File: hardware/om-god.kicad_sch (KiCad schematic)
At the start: 0 parts

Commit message: fd
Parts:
- added C1: 100nF, Capacitor_SMD:C_0402_1005Metric, symbol Device:C
- added C44, C55, C59, C60, C61, C62, C70, C71: 10uF, Capacitor_SMD:C_0402_1005Metric, symbol Device:C
- added C45: 22uF, Capacitor_SMD:C_0402_1005Metric, symbol Device:C
- added C56, C65, C66: 1uF, Capacitor_SMD:C_0402_1005Metric, symbol Device:C
- added C57, C69: 4.7uF, Capacitor_SMD:C_0402_1005Metric, symbol Device:C
- added C58: 47nF, Capacitor_SMD:C_0402_1005Metric, symbol Device:C
- added C63, C67, C68: 2.2uF, Capacitor_SMD:C_0402_1005Metric, symbol Device:C
- added C64: 470nF, Capacitor_SMD:C_0402_1005Metric, symbol Device:C
- added CN1: USB-B-Female-90, lcsc:USB-B_TH_USB-B-FEMALE-90, symbol lcsc:USB-B-Female-90
- added CN2, CN3: DIN-504B-M10, lcsc:CONN-TH_DIN-504B-M10, symbol lcsc:DIN-504B-M10
- added CN4: PJ-320D, lcsc:AUDIO-SMD_PJ-320D, symbol lcsc:PJ-320D
- added Card1: TF PUSH, lcsc:TF-SMD_TF-PUSH, symbol lcsc:TFPUSH
- added D1, D10, D11, D12, D13, D14, D15, D16, D17, D18, D19, D2, D20, D21, D22, D23, D24, D25, D3, D4, D5, D50, D51, D52, D53, D54, D55, D56, D57, D58, D59, D6, D60, D61, D62, D63, D64, D65, D66, D67, D68, D69, D7, D70, D71, D72, D8, D9: 1N4148WS_C917117, lcsc:SOD-323_L1.8-W1.3-LS2.5-RD, symbol lcsc:1N4148WS_C917117
- added D26: 1N4148WT, Diode_SMD:D_SOD-523, symbol Diode:1N4148WT
- added D27: PESD15VL1BA, PCM_Diode_SMD_AKL:D_SOD-323_TVS, symbol PCM_Diode_TVS_AKL:PESD15VL1BA
- added FPC1: 5034801200, lcsc:FPC-SMD_5034801200, symbol lcsc:5034801200
- added J1, J2: Conn_01x13_Pin, symbol Connector:Conn_01x13_Pin
- added J3, J4, J5: PJ-625G, lcsc:AUDIO-TH_PJ-625G, symbol lcsc:PJ-625G
- added J6, J7: Conn_01x01_Pin, symbol Connector:Conn_01x01_Pin
- added J8: Conn_01x03, Connector_JST:JST_EH_S3B-EH_1x03_P2.50mm_Horizontal, symbol Connector_Generic:Conn_01x03
- added L4: 1uH, Inductor_SMD:L_0603_1608Metric, symbol Device:L
- added L5, L6: 470nH, Inductor_SMD:L_0603_1608Metric, symbol Device:L
- added L8: EXC14CE900U, linea:FILTER-SMD_4P-L0.9-W0.7-P0.50-BL, symbol linea:EXC14CE900U
- added L9: 470nH, Inductor_SMD:L_Murata_DFE201610P, symbol Device:L
- added Q4: ~, linea:SOT-523-3_L1.6-W0.8-P1.00-LS1.6-BR, symbol DMN313DLT-7:DMN313DLT-7
- added Q5: ~, linea:SOT-363_L2.0-W1.3-P0.65-LS2.1-BL, symbol MMDT2907A-7-F:MMDT2907A-7-F
- added Q6: ~, linea:SOT-23-3_L2.9-W1.3-P1.90-LS2.4-BR, symbol DMP1045U-7:DMP1045U-7
- added R1, R2: 5.1K, Resistor_SMD:R_0402_1005Metric, symbol Device:R
- added R31, R32: 1.5K, Resistor_SMD:R_0402_1005Metric, symbol Device:R
- added R33: 4.7K, Resistor_SMD:R_0402_1005Metric, symbol Device:R
- added R34, R36, R40, R41: 10K, Resistor_SMD:R_0402_1005Metric, symbol Device:R
- added R35: 100, Resistor_SMD:R_0402_1005Metric, symbol Device:R
- added R37: 470, Resistor_SMD:R_0402_1005Metric, symbol Device:R
- added R38: 30.1K, Resistor_SMD:R_0402_1005Metric, symbol Device:R
- added R39: 5.23K, Resistor_SMD:R_0402_1005Metric, symbol Device:R
- added R42: 10m, Resistor_SMD:R_0402_1005Metric, symbol Device:R
- added R43: DNP, Resistor_SMD:R_0402_1005Metric, symbol Device:R
- added R44, R45: 1.5, Resistor_SMD:R_0402_1005Metric, symbol Device:R
- added R46, R47: 3.3, Resistor_SMD:R_0402_1005Metric, symbol Device:R
- added R48, R49: 100K, Resistor_SMD:R_0402_1005Metric, symbol Device:R
- added SW1, SW10, SW11, SW12, SW13, SW14, SW15, SW16, SW17, SW18, SW19, SW2, SW20, SW21, SW22, SW23, SW24, SW25, SW26, SW27, SW28, SW29, SW3, SW30, SW31, SW32, SW33, SW34, SW35, SW36, SW37, SW38, SW39, SW4, SW40, SW41, SW42, SW43, SW44, SW45, SW46, SW47, SW48, SW5, SW56, SW57, SW58, SW6, SW7, SW8, SW9: TS-1003ST-26, lcsc:SW-SMD_4P-L12.0-W12.0-P5.00-LS15.4, symbol lcsc:TS-1003ST-26
- added SW49: RotaryEncoder_Switch, symbol Device:RotaryEncoder_Switch
- added SW50, SW51, SW52, SW53, SW54, SW55: RotaryEncoder, symbol Device:RotaryEncoder
- added TP1, TP2, TP3: TestPoint, TestPoint:TestPoint_Pad_1.5x1.5mm, symbol Connector:TestPoint
- added U1: TDA7297, Package_TO_SOT_THT:TO-220-15_P2.54x2.54mm_StaggerOdd_Lead4.58mm_Vertical, symbol Amplifier_Audio:TDA7297
- added U10, U11, U7, U8, U9: ~, lcsc:SW-TH_6P-L8.0-W8.0-P2.50, symbol lcsc:XKB8080-Z
- added U12: ~, linea:DSBGA-6_L1.4-W1.1-R3-C2-P0.40-BL, symbol LM3281YFQR:LM3281YFQR
- added U13: ~, linea:QFN-24_L4.0-W4.0-P0.50-TL-EP2.7, symbol BQ25896RTWR:BQ25896RTWR
- added U14: ~, linea:DSBGA-9_L1.7-W1.6-R3-C3-P0.50-BL, symbol BQ27220YZFR:BQ27220YZFR
- added U15: FAN48610BUC50X, linea:WLCSP-9_L1.2-W1.2-R3-C3-P0.40-BL, symbol linea:FAN48610BUC50X
- added U16: RS3221-3.3YUTDN4, linea:UTDFN-4_L1.0-W1.0-P0.63-BL-EP-1, symbol linea:RS3221-3.3YUTDN4
- added U17: USBLC6-2P6, Package_TO_SOT_SMD:SOT-666, symbol Power_Protection:USBLC6-2P6
- added U2: TPA3116D2DAD_C2865736, lcsc:HTSSOP-32_L11.0-W6.1-P0.65-LS8.1-BL, symbol lcsc:TPA3116D2DAD_C2865736
- added U3: CY8CMBR3116-LQXIT, lcsc:QFN-24_L4.0-W4.0-P0.50-BL-EP2.6, symbol lcsc:CY8CMBR3116-LQXIT
- added U4: PCM5102APWR, lcsc:TSSOP-20_L6.5-W4.4-P0.65-LS6.4-BL, symbol lcsc:PCM5102APWR
- added U5: HS20HS072RX, lcsc:OLED-SMD_HS20HS072RX, symbol lcsc:HS20HS072RX
- added U6: MKDV4GCL-ABB, lcsc:LGA-8_L6.0-W8.0-P1.27-TL, symbol lcsc:MKDV4GCL-ABB
- added USB2: TYPE-C 16PIN 2MD(073), linea:USB-C-SMD_TYPE-C-6PIN-2MD-073, symbol linea:TYPE-C16PIN2MD(073)
- added VQ: STM32H723ZGT6, lcsc:LQFP-144_L20.0-W20.0-P0.50-LS22.0-BL, symbol lcsc:STM32H723ZGT6
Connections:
- new net: D72.2 (A), SW23.1, SW23.2
- new net: D52.2 (A), SW2.1, SW2.2
- new net: D70.2 (A), SW21.1, SW21.2
- new net: D21.2 (A), SW44.1, SW44.2
- new net: D3.2 (A), SW26.1, SW26.2
- new net: D60.2 (A), SW10.1, SW10.2
- new net: D65.2 (A), SW16.1, SW16.2
- new net: D2.2 (A), SW24.1, SW24.2
- new net: D19.2 (A), SW42.1, SW42.2
- new net: L8.3, U17.6 (I/O1)
- new net: L8.4, U17.4 (I/O2)
- new net: D57.2 (A), SW7.1, SW7.2
- new net: Q5.3 (C2), R48.1
- new net: D24.2 (A), SW47.1, SW47.2
- new net: D63.2 (A), SW14.1, SW14.2
- new net: C68.1, C69.1, C70.1, L6.1, R44.1, R45.1, U12.A1 (FB)
- new net: L5.1, U12.B2 (SW)
- new net: L6.2, R46.2, R47.2
- new net: L5.2, R44.2, R45.2
- new net: D5.2 (A), SW28.1, SW28.2
- new net: D61.2 (A), SW11.1, SW11.2
- new net: D9.2 (A), SW32.1, SW32.2
- new net: D56.2 (A), SW6.1, SW6.2
- new net: D64.2 (A), SW15.1, SW15.2
- new net: D12.2 (A), SW35.1, SW35.2
- new net: L9.2, U15.B1 (SW), U15.B2 (SW)
- new net: D20.2 (A), SW43.1, SW43.2
- new net: D17.2 (A), SW40.1, SW40.2
- new net: R37.2, U13.10 (LIIM)
- new net: J8.2 (Pin_2), R38.2, R39.2, R43.1, TP2.1, U13.11 (TS)
- new net: C61.1, C62.1, C66.1, R42.2, U13.13 (BAT), U13.14 (BAT), U14.C2 (SRN), U16.3 (EN), U16.4 (IN)
- new net: C58.1, L4.1, U13.19 (SW), U13.20 (SW)
- new net: C58.2, U13.21 (BTST)
- new net: C57.1, R39.1, U13.22 (REGN)
- new net: C55.1, U13.23 (PMID)
- new net: R33.1, U13.7 (INT)
- new net: Q4.3 (D), R34.1, U13.8 (OTG)
- new net: D13.2 (A), SW36.1, SW36.2
- new net: Q4.1 (G), R35.1, R36.2
- new net: D62.2 (A), SW12.1, SW12.2
- new net: D55.2 (A), SW5.1, SW5.2
- new net: D51.2 (A), SW25.1, SW25.2
- new net: D16.2 (A), SW39.1, SW39.2
- new net: D23.2 (A), SW46.1, SW46.2
- new net: D7.2 (A), SW30.1, SW30.2
- new net: R2.1, USB2.10 (CC2)
- new net: D11.2 (A), SW34.1, SW34.2
- new net: D68.2 (A), SW19.1, SW19.2
- new net: D14.2 (A), SW37.1, SW37.2
- new net: D15.2 (A), SW38.1, SW38.2
- new net: D8.2 (A), SW31.1, SW31.2
- new net: D54.2 (A), SW4.1, SW4.2
- new net: D53.2 (A), SW3.1, SW3.2
- new net: R40.1, U14.A1 (GPOUT)
- new net: R41.2, U14.B1 (BIN)
- new net: C63.1, C64.1, U14.B3 (VDD)
- new net: D66.2 (A), SW17.1, SW17.2
- new net: D18.2 (A), SW41.1, SW41.2
- new net: D22.2 (A), SW45.1, SW45.2
- new net: D50.2 (A), SW13.1, SW13.2
- new net: D26.2 (A), Q5.2 (B1), Q5.5 (B2)
- new net: Q5.6 (C1), Q6.1 (G), R49.1
- new net: D67.2 (A), SW18.1, SW18.2
- new net: D25.2 (A), SW48.1, SW48.2
- new net: D59.2 (A), SW9.1, SW9.2
- new net: U17.1 (I/O1), USB2.6 (DP1), USB2.8 (DP2)
- new net: U17.3 (I/O2), USB2.5 (DN2), USB2.7 (DN1)
- new net: D1.2 (A), SW1.1, SW1.2
- new net: D10.2 (A), SW33.1, SW33.2
- new net: D58.2 (A), SW8.1, SW8.2
- new net: R1.1, USB2.4 (CC1)
- new net: D6.2 (A), SW29.1, SW29.2
- new net: D71.2 (A), SW22.1, SW22.2
- new net: D69.2 (A), SW20.1, SW20.2
- new net: D4.2 (A), SW27.1, SW27.2
- new net +3.3V: C71.1, R31.2, R32.2, R33.2, R40.2, R46.1, R47.1
- new net +5V: C45.1, U15.A1 (VOUT), U15.A2 (VOUT)
- new net +BATT: C65.1, J8.1 (Pin_1), R42.1, TP1.1, U14.C1 (SRP), U14.C3 (BAT)
- new net 7th: D10.1 (C), D12.1 (C), D14.1 (C), D16.1 (C), D18.1 (C), D2.1 (C), D20.1 (C), D22.1 (C), D24.1 (C), D4.1 (C), D6.1 (C), D8.1 (C)
- new net Chord A: SW1.3, SW1.4, SW11.3, SW11.4, SW24.3, SW24.4, SW26.3, SW26.4
- new net Chord Ab: SW10.3, SW10.4, SW23.3, SW23.4, SW47.3, SW47.4, SW48.3, SW48.4
- new net Chord B: SW14.3, SW14.4, SW25.3, SW25.4, SW29.3, SW29.4, SW30.3, SW30.4
- new net Chord Bb: SW12.3, SW12.4, SW13.3, SW13.4, SW27.3, SW27.4, SW28.3, SW28.4
- new net Chord C: SW15.3, SW15.4, SW2.3, SW2.4, SW31.3, SW31.4, SW32.3, SW32.4
- new net Chord D: SW17.3, SW17.4, SW35.3, SW35.4, SW36.3, SW36.4, SW4.3, SW4.4
- new net Chord Db: SW16.3, SW16.4, SW3.3, SW3.4, SW33.3, SW33.4, SW34.3, SW34.4
- new net Chord E: SW19.3, SW19.4, SW39.3, SW39.4, SW40.3, SW40.4, SW6.3, SW6.4
- new net Chord Eb: SW18.3, SW18.4, SW37.3, SW37.4, SW38.3, SW38.4, SW5.3, SW5.4
- new net Chord F: SW20.3, SW20.4, SW41.3, SW41.4, SW42.3, SW42.4, SW7.3, SW7.4
- new net Chord G: SW22.3, SW22.4, SW45.3, SW45.4, SW46.3, SW46.4, SW9.3, SW9.4
- new net Chord Gb: SW21.3, SW21.4, SW43.3, SW43.4, SW44.3, SW44.4, SW8.3, SW8.4
- new net Extention: D11.1 (C), D13.1 (C), D15.1 (C), D17.1 (C), D19.1 (C), D21.1 (C), D23.1 (C), D25.1 (C), D3.1 (C), D5.1 (C), D7.1 (C), D9.1 (C)
- new net GND: C1.2, C44.2, C45.2, C55.2, C56.2, C57.2, C59.2, C60.2, C61.2, C62.2, C63.2, C64.2, C65.2, C66.2, C67.2, C68.2, C69.2, C70.2, C71.2, D27.1 (K), J8.3 (Pin_3), Q4.2 (S), R1.2, R2.2, R36.1, R37.1, R38.1, R41.1, R43.2, R48.2, R49.2, TP3.1, U12.C2 (GND), U13.17 (PGND), U13.18 (PGND), U13.2 (PSEL), U13.25 (EPAD), U13.9 (CE), U14.B2 (VSS), U15.C1 (PGND), U15.C2 (PGND), U15.C3 (AGND), U16.2 (GND), U16.5 (EP), U17.2 (GND), USB2.1 (GND), USB2.12 (GND), USB2.13 (SHELL), USB2.14 (SHELL)
- new net I2C_SCL: R31.1, U13.5 (SCL), U14.A3 (SCL)
- new net I2C_SDA: R32.1, U13.6 (SDA), U14.A2 (SDA)
- new net LDO_3.3V: U16.1 (OUT)
- new net Mayor: D1.1 (C), D50.1 (C), D51.1 (C), D52.1 (C), D53.1 (C), D54.1 (C), D55.1 (C), D56.1 (C), D57.1 (C), D58.1 (C), D59.1 (C), D60.1 (C)
- new net Minor: D61.1 (C), D62.1 (C), D63.1 (C), D64.1 (C), D65.1 (C), D66.1 (C), D67.1 (C), D68.1 (C), D69.1 (C), D70.1 (C), D71.1 (C), D72.1 (C)
- new net RESET: U13.12 (QON)
- new net SYS: C44.1, C59.1, C60.1, C67.1, L4.2, L9.1, R34.2, U12.A2 (VIN), U12.B1 (MODE), U12.C1 (EN), U13.15 (SYS), U13.16 (SYS), U15.A3 (VIN), U15.B3 (EN)
- new net USB_5V: C56.1, Q5.4 (E2), Q6.2 (S), U13.1 (VBUS)
- new net VBUS: C1.1, D26.1 (K), D27.2 (A), Q5.1 (E1), Q6.3 (D), R35.2, U17.5 (VBUS), USB2.11 (VBUS), USB2.2 (VBUS)
- no-connect marks 0 -> 3
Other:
- note added: "Advanced Funtionalities"
- note added: "Audio Amplifiers"
- note added: "Audio Out"
- note added: "Chord Matrix"
- note added: "Chords Volume"
- note added: "DAC"
- note added: "DIN-MIDI"
- note added: "External Micro SD Card"
- note added: "Function Knob"
- note added: "Headphones Out"
- note added: "I/O"
- note added: "If using thermistor, remove R43"
- note added: "Instant Off"
- note added: "Keyboard Volume"
- note added: "Main"
- note added: "Main Buttons"
- note added: "Main Knobs"
- note added: "Main Volume"
- note added: "Metronome"
- note added: "Midi"
- note added: "NAnd Flash"
- note added: "Next Chord"
- note added: "Octave Down"
- note added: "Octave Up"
- note added: "On/Off"
- note added: "Pedal"
- note added: "Power Managment"
- note added: "Recording"
- note added: "Recording Mode"
- note added: "Rythm"
- note added: "Rythm Volume"
- note added: "Sonic Strings"
- note added: "Stereo Out"
- note added: "Sustain Chord"
- note added: "Touch Pad"
- note added: "Touch Pad Volume"
- note added: "USB-MIDI"
- note added: "Usb Power outlet / Coding"
- note added: "VQ"
- note added: "Vibrato Knob"
- note added: "Volume"

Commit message: yes
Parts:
- removed CN4: PJ-320D, lcsc:AUDIO-SMD_PJ-320D, symbol lcsc:PJ-320D
- removed D26: 1N4148WT, Diode_SMD:D_SOD-523, symbol Diode:1N4148WT
- removed J2: Conn_01x13_Pin, symbol Connector:Conn_01x13_Pin
- removed J6, J7: Conn_01x01_Pin, symbol Connector:Conn_01x01_Pin
- removed J8: Conn_01x03, Connector_JST:JST_EH_S3B-EH_1x03_P2.50mm_Horizontal, symbol Connector_Generic:Conn_01x03
- removed L9: 470nH, Inductor_SMD:L_Murata_DFE201610P, symbol Device:L
- removed Q4: ~, linea:SOT-523-3_L1.6-W0.8-P1.00-LS1.6-BR, symbol DMN313DLT-7:DMN313DLT-7
- removed Q5: ~, linea:SOT-363_L2.0-W1.3-P0.65-LS2.1-BL, symbol MMDT2907A-7-F:MMDT2907A-7-F
- removed Q6: ~, linea:SOT-23-3_L2.9-W1.3-P1.90-LS2.4-BR, symbol DMP1045U-7:DMP1045U-7
- removed TP1, TP2, TP3: TestPoint, TestPoint:TestPoint_Pad_1.5x1.5mm, symbol Connector:TestPoint
- removed U1: TDA7297, Package_TO_SOT_THT:TO-220-15_P2.54x2.54mm_StaggerOdd_Lead4.58mm_Vertical, symbol Amplifier_Audio:TDA7297
- removed U12: ~, linea:DSBGA-6_L1.4-W1.1-R3-C2-P0.40-BL, symbol LM3281YFQR:LM3281YFQR
- removed U13: ~, linea:QFN-24_L4.0-W4.0-P0.50-TL-EP2.7, symbol BQ25896RTWR:BQ25896RTWR
- removed U14: ~, linea:DSBGA-9_L1.7-W1.6-R3-C3-P0.50-BL, symbol BQ27220YZFR:BQ27220YZFR
- removed U15: FAN48610BUC50X, linea:WLCSP-9_L1.2-W1.2-R3-C3-P0.40-BL, symbol linea:FAN48610BUC50X
- removed U16: RS3221-3.3YUTDN4, linea:UTDFN-4_L1.0-W1.0-P0.63-BL-EP-1, symbol linea:RS3221-3.3YUTDN4
- removed U4: PCM5102APWR, lcsc:TSSOP-20_L6.5-W4.4-P0.65-LS6.4-BL, symbol lcsc:PCM5102APWR
- added AUDIO1: PJ-393_C2837065, lcsc:AUDIO-SMD_PJ-393, symbol lcsc:PJ-393_C2837065
- added C10, C104, C12, C133, C134, C135, C136, C142, C143, C145, C146, C148, C155, C156, C157, C158, C167, C177, C179, C180, C181, C185, C186, C189, C19, C194, C20, C3, C4, C41, C42, C43, C46, C47, C48, C49, C5, C51, C52, C53, C54, C6, C7, C8, C82, C83, C84, C86, C9, C94, C96: 0.1uF, symbol Device:C
- added C105, C106, C107, C120, C121, C124, C127, C128, C166, C22, C23, C24, C32, C33, C34, C35, C50, C95: 1uF, symbol Device:C
- added C108, C109, C21, C25, C38: 1nF, symbol Device:C
- added C11, C18, C188, C191, C195, C196, C2, C80, C81, C85, C92, C93, C97: 2.2uF, symbol Device:C
- added C110, C111, C112, C113, C165, C28, C29, C30, C31: 220nF, symbol Device:C
- added C114, C115, C131, C26, C39: 100nF, symbol Device:C
- added C116, C117, C27, C40: 220uF, symbol Device:C_Polarized
- added C118, C119, C125, C126: 680nF, symbol Device:C
- added C122, C123, C129, C130, C132, C36, C37: 10nF, symbol Device:C
- added C13, C14, C147, C15, C150, C152, C153, C16, C17, C184, C187, C190, C192, C193, C87, C88, C89, C90, C91: 10uF, symbol Device:C_Polarized
- added C137, C138: 220pF, Capacitor_SMD:C_0402_1005Metric, symbol Device:C
- added C139: 0.1uF, Capacitor_SMD:C_0402_1005Metric, symbol Device:C
- added C140, C149, C151: 1uF, symbol Device:C_Polarized
- added C141: 0.056uF, symbol Device:C_Polarized
- added C144: 2.2uF, symbol Device:C_Polarized
- added C154: 22pF, symbol Device:C
- added C159, C168: 47pF, symbol Device:C
- added C160, C161, C162, C163, C169, C170, C171, C172, C173, C174, C182, C183: 22uF, symbol Device:C
- added C164, C175, C176, C178: 10uF, symbol Device:C
- added C72, C73, C75, C77: 82nF, PCM_Capacitor_THT_AKL:C_Rect_L4.0mm_W2.5mm_P2.50mm, symbol PCM_Capacitor_AKL:C_Rect_L4.0mm_W2.5mm_P2.50mm
- added C74, C76, C78, C79: 5.6nF, PCM_Capacitor_THT_AKL:C_Rect_L4.0mm_W2.5mm_P2.50mm, symbol PCM_Capacitor_AKL:C_Rect_L4.0mm_W2.5mm_P2.50mm
- added D28: BAT54, PCM_Package_TO_SOT_SMD_AKL:SOT-23, symbol PCM_Diode_Schottky_AKL:BAT54
- added D29, D30, D31: LED, symbol Device:LED
- added J2: Conn_01x03_Pin, symbol Connector:Conn_01x03_Pin
- added L1, L10, L11, L2, L3, L7: 10uH, symbol Device:L
- added L12: 6.8uH, Inductor_SMD:L_6.3x6.3_H3, symbol Device:L
- added L13: 6.8uH, symbol Device:L
- added L14: 15uH, symbol Device:L
- added Q1, Q2, Q3: Si7617DN, Package_SO:Vishay_PowerPAK_1212-8_Single, symbol Transistor_FET:Si7617DN
- added R10, R13, R17, R18, R26: 100k, symbol Device:R
- added R100, R101, R87, R99: 10K, Resistor_SMD:R_0402_1005Metric, symbol Device:R
- added R102, R66, R69, R74: 100K, Resistor_SMD:R_0402_1005Metric, symbol Device:R
- added R103: NTCG163JF103FT1S, lcsc:R0603, symbol lcsc:NTCG163JF103FT1S
- added R104: 9.31K, Resistor_SMD:R_0402_1005Metric, symbol Device:R
- added R105: 430K, Resistor_SMD:R_0402_1005Metric, symbol Device:R
- added R11, R16: 75k, symbol Device:R
- added R12, R9: 47k, symbol Device:R
- added R14, R15, R19, R20, R24, R25: 3.3, symbol Device:R
- added R21, R22, R27, R28, R29, R30, R50, R51, R52, R53, R7, R8, R82, R83, R84, R85: 10K, symbol Device:R
- added R23: 10k, symbol Device:R
- added R3, R4: 470K, symbol Device:R
- added R5, R59, R6, R60, R61, R62, R63, R64, R65, R67, R68, R70, R71, R72, R73, R75: 6K, symbol Device:R
- added R58: 200K, Resistor_SMD:R_0402_1005Metric, symbol Device:R
- added R76, R77, R78, R79, R80, R81, R89, R94: 1K, symbol Device:R
- added R86: 22.1K, Resistor_SMD:R_0402_1005Metric, symbol Device:R
- added R88: 32.4K, Resistor_SMD:R_0402_1005Metric, symbol Device:R
- added R90, R95, R98: 100K, symbol Device:R
- added R91: 10, symbol Device:R
- added R92: 2, symbol Device:R
- added R93, R96: 0.01, symbol Device:R
- added R97: 500K, symbol Device:R
- added U1, U18, U19, U20, U22, U24, U25, U28, U29: NE5532DR, lcsc:SOIC-8_L4.9-W3.9-P1.27-LS6.0-BL, symbol lcsc:NE5532DR
- added U12, U13, U14, U35: LMR33630ADDAR, lcsc:ESOP-8_L4.9-W3.9-P1.27-LS6.0-TL-EP, symbol lcsc:LMR33630ADDAR
- added U15: TPS54202DDC, Package_TO_SOT_SMD:SOT-23-6, symbol Regulator_Switching:TPS54202DDC
- added U16, U26, U4: PCM5122PW, Package_SO:TSSOP-28_4.4x9.7mm_P0.65mm, symbol Audio:PCM5122PW
- added U21: TPA6120A2DWP, lcsc:HSOP-20_L12.8-W7.5-P1.27-LS10.3-BL-EP3.3, symbol lcsc:TPA6120A2DWP
- added U23: TS5A23159RSER, lcsc:UQFN-10_L2.0-W1.5-P0.50-BL-EP, symbol lcsc:TS5A23159RSER
- added U30: TPA3116D2DAD_C2865736, lcsc:HTSSOP-32_L11.0-W6.1-P0.65-LS8.1-BL, symbol lcsc:TPA3116D2DAD_C2865736
- added U31: BQ24610, Package_DFN_QFN:VQFN-24-1EP_4x4mm_P0.5mm_EP2.45x2.45mm, symbol Battery_Management:BQ24610
- added U32: TUSB422IYFPR, lcsc:DSBGA-9_L1.4-W1.3-R3-C3-P0.40-BL, symbol lcsc:TUSB422IYFPR
- added U33, U34: SIS412DN-T1-GE3-ES, lcsc:PDFN-8_L3.1-W3.1-P0.65-LS3.4-BL, symbol lcsc:SIS412DN-T1-GE3-ES
- C44, C66: footprint Capacitor_SMD:C_0402_1005Metric -> (none)
- C45: value 22uF -> 220nF; footprint Capacitor_SMD:C_0402_1005Metric -> (none)
- C55: value 10uF -> 0.1uF; footprint Capacitor_SMD:C_0402_1005Metric -> (none)
- C56: value 1uF -> 47pF; footprint Capacitor_SMD:C_0402_1005Metric -> (none); now not fitted
- C57: value 4.7uF -> 22uF; footprint Capacitor_SMD:C_0402_1005Metric -> (none)
- C58: value 47nF -> 22uF; footprint Capacitor_SMD:C_0402_1005Metric -> (none)
- C59, C60, C70, C71: value 10uF -> 22uF; footprint Capacitor_SMD:C_0402_1005Metric -> (none)
- C61: value 10uF -> 1uF; footprint Capacitor_SMD:C_0402_1005Metric -> (none)
- C62: value 10uF -> 220nF; footprint Capacitor_SMD:C_0402_1005Metric -> (none)
- C63: value 2.2uF -> 10uF; footprint Capacitor_SMD:C_0402_1005Metric -> (none)
- C64: value 470nF -> 10uF; footprint Capacitor_SMD:C_0402_1005Metric -> (none)
- C65: value 1uF -> 220nF; footprint Capacitor_SMD:C_0402_1005Metric -> (none)
- C67: value 2.2uF -> 1uF; footprint Capacitor_SMD:C_0402_1005Metric -> (none)
- C68: value 2.2uF -> 0.1uF; footprint Capacitor_SMD:C_0402_1005Metric -> (none)
- C69: value 4.7uF -> 47pF; footprint Capacitor_SMD:C_0402_1005Metric -> (none); now not fitted
- L4: value 1uH -> 8uH; footprint Inductor_SMD:L_0603_1608Metric -> (none)
- L5: value 470nH -> 15uH; footprint Inductor_SMD:L_0603_1608Metric -> (none)
- L6: value 470nH -> 27uH; footprint Inductor_SMD:L_0603_1608Metric -> (none)
- R1, R2: value 5.1K -> 1.5K
- R31: value 1.5K -> 100K
- R32: value 1.5K -> 24.9K
- R33: value 4.7K -> 100K
- R34, R40, R41: value 10K -> 100K
- R35: value 100 -> 100K
- R36: value 10K -> 43.2K
- R37: value 470 -> 100K
- R38: value 30.1K -> 100K
- R39: value 5.23K -> 9.09K
- R42: value 10m -> 9.09K
- R43: value DNP -> 49.9
- R44: value 1.5 -> 50k
- R45: value 1.5 -> 2.61k
- R46, R47: value 3.3 -> 470K; footprint Resistor_SMD:R_0402_1005Metric -> (none)
- R48, R49: value 100K -> 470K; footprint Resistor_SMD:R_0402_1005Metric -> (none)
- renumbered VQ to VQ1
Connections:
- net I2C_SDA is gone; now on net GND: R32.1
- net USB_5V is gone; now on net +5V: C56.1
- net +3.3V: now also R1.1, R2.2, R35.2, U3.7 (VDD), C139.1, C15.1, C159.1, C160.1, C161.1, C162.1, C163.1, C184.1, C185.1, C49.1, C83.1, C89.1, C9.1, C94.1, C95.1, L13.2, R104.1, R58.1, R66.2, R69.2, R74.2, R82.1, R83.1, R84.2, R85.2, U16.17 (MODE1), U16.28 (DVDD), U23.8 (VCC), U26.17 (MODE1), U26.28 (DVDD), U32.A3 (VDD), U4.17 (MODE1), U4.28 (DVDD); no longer C71.1, R31.2, R32.2, R33.2, R40.2, R46.1, R47.1
- net +5V: now also C57.1, C58.1, C59.1, C60.1, L4.2, R31.2; no longer C45.1
- net +BATT: now also C152.1, C153.1, C154.2, C155.1, Q3.5 (D), R96.2, R97.1, U31.13 (SRN); no longer C65.1, R42.1
- net GND: now also C58.2, J3.2, J4.2, L6.2, R39.1, R42.1, U2.1 (MODSEL), U2.10 (LINP), U2.11 (LINN), U2.13 (AM2), U2.14 (AM1), U2.15 (AM0), U2.22 (GND), U2.25 (GND), U2.28 (GND), U2.33 (PAD), U2.9 (GND), U3.8 (VSS), AUDIO1.4, C10.1, C104.1, C108.1, C109.1, C11.1, C114.1, C115.1, C116.2, C117.2, C118.1, C119.2, C12.2, C120.1, C121.2, C122.1, C123.2, C125.1, C126.2, C127.1, C128.2, C129.1, C13.2, C130.2, C131.1, C132.2, C133.1, C134.2, C135.2, C136.1, C137.2, C138.2, C139.2, C14.2, C140.2, C141.2, C144.2, C146.1, C147.2, C149.2, C15.2, C150.2, C151.2, C152.2, C153.2, C156.2, C157.2, C16.2, C160.2, C161.2, C162.2, C163.2, C164.2, C165.2, C166.2, C169.2, C17.2, C170.2, C171.2, C172.2, C173.2, C174.2, C175.2, C176.2, C177.2, C18.2, C181.1, C182.1, C183.1, C184.2, C185.2, C186.1, C187.2, C188.1, C189.2, C19.1, C190.2, C192.2, C193.2, C194.2, C195.2, C196.2, C20.1, C21.2, C22.2, C25.1, C26.1, C27.2, C3.2, C32.2, C33.1, C34.1, C35.2, C36.1, C37.2, C38.1, C39.1, C4.1, C40.2, C41.1, C42.1, C43.1, C46.1, C47.1, C48.1, C49.2, C5.1, C50.2, C51.1, C52.1, C53.1, C54.1, C6.1, C7.1, C72.1, C73.1, C78.1, C79.1, C8.1, C80.2, C82.2, C83.2, C84.1, C85.1, C86.2, C87.2, C88.2, C89.2, C9.2, C90.2, C91.2, C92.2, C93.2, C94.2, C95.2, C96.2, C97.2, R10.2, R103.2, R105.2, R11.2, R16.2, R18.2, R29.1, R30.1, R50.1, R51.1, R6.2, R60.2, R65.2, R68.2, R73.2, R77.1, R81.1, R86.2, R87.2, R88.2, R98.2, U12.1 (PGND), U12.9 (EP), U13.1 (PGND), U13.9 (EP), U14.1 (PGND), U14.9 (EP), U16.18 (MODE2/MS), U16.27 (DGND), U16.3 (CPGND), U16.9 (AGND), U18.4 (IN2+), U18.6 (IN1+), U20.4 (IN2+), U20.6 (IN1+), U22.6 (IN1+), U23.3 (GND), U26.18 (MODE2/MS), U26.27 (DGND), U26.3 (CPGND), U26.9 (AGND), U30.1 (MODSEL), U30.13 (AM2), U30.14 (AM1), U30.15 (AM0), U30.22 (GND), U30.25 (GND), U30.28 (GND), U30.33 (PAD), U30.9 (GND), U31.17 (GND), U31.25 (GND), U32.C2 (GND), U34.1 (S), U34.2 (S), U34.3 (S), U35.1 (PGND), U35.9 (EP), U4.18 (MODE2/MS), U4.27 (DGND), U4.3 (CPGND), U4.9 (AGND); no longer C55.2, C56.2, C68.2, C69.2, R1.2, R2.2, R37.1, R38.1, R41.1, R48.2, R49.2
- net SYS: now also C45.1, C62.1, C63.1, C64.1, C65.1, C145.2, C147.1, C148.2, C150.1, C164.1, C165.1, Q3.1 (S), Q3.2 (S), Q3.3 (S), R93.2, R95.1, U12.2 (VIN), U12.3 (EN), U13.2 (VIN), U13.3 (EN), U14.2 (VIN), U14.3 (EN), U31.1 (ACN), U33.5 (D), U33.6 (D), U33.7 (D), U33.8 (D), U33.9 (D), U35.2 (VIN), U35.3 (EN); no longer C59.1, C60.1, C67.1, L4.2, R34.2
- net VBUS: now also Q1.5 (D), R100.2, R101.2, R92.2, R99.2, U32.A2 (VBUSIN); no longer R35.2
- net DN USB: now reaches L8.1
- net DP USB: now reaches L8.2
- net at R48.1: now also U26.6 (OUTL)
- net at L5.1: now also C68.1, U12.8 (SW)
- net STEREO BUFF L/MONO: now reaches J4.6
- net STEREO BUFF L/MONO: now also U23.10 (COM1)
- net STEREO GPIO L/MONO: now reaches J4.7
- net STEREO GPIO L/MONO: now also R83.2
- net PG: now reaches R37.2
- net PG: now also R33.2, R34.2, R40.2, U12.4 (PG), U13.4 (PG), U14.4 (PG), U35.4 (PG)
- net at L4.1: now also C55.1, U35.8 (SW); no longer C58.1
- net at R33.1: now also C61.1, U35.6 (VCC)
- net at R34.1: now also C66.1, U13.6 (VCC)
- net at R35.1, R36.2: now also C159.2, U13.5 (FB)
- net STEREO BUFF R: now reaches J3.6
- net STEREO BUFF R: now also U1.2 (OUT2), U1.3 (IN2-)
- net STEREO GPIO R: now reaches J3.7
- net STEREO GPIO R: now also R82.2
- net at USB2.10 (CC2): now also C137.1, U32.A1 (CC2); no longer R2.1
- net MUTE SUB: now reaches U2.12 (MUTE)
- net MUTE SUB: now also R10.1
- net at U2.16 (SYNC): now also C21.1, R23.2
- net +12V: now reaches U2.17 (AVCC)
- net +12V: now also C69.1, C70.1, C71.1, L5.2, R38.2, R41.2, U2.18 (PVCC), U2.19 (PVCC), U2.31 (PVCC), U2.32 (PVCC), C104.2, C108.2, C109.2, C114.2, C115.2, C116.1, C117.1, C132.1, C134.1, C135.1, C168.1, C169.1, C170.1, C171.1, C172.1, C173.1, C174.1, C175.1, C176.1, C177.1, C178.1, C179.1, C20.2, C25.2, C26.2, C27.1, C38.2, C39.2, C40.1, C42.2, C43.2, C47.2, C5.2, C52.2, C54.2, C7.2, L14.2, R13.1, R17.1, R26.2, R61.2, U1.1 (VCC+), U15.3 (VIN), U18.1 (VCC+), U19.1 (VCC+), U20.1 (VCC+), U21.18 (RVCC+), U21.3 (LVCC+), U22.1 (VCC+), U24.1 (VCC+), U25.1 (VCC+), U28.1 (VCC+), U29.1 (VCC+), U30.17 (AVCC), U30.18 (PVCC), U30.19 (PVCC), U30.31 (PVCC), U30.32 (PVCC)
- net /SD SUB: now reaches U2.2 (SDZ)
- net /SD SUB: now also U2.3 (FAULTZ), R13.2
- net at U2.20 (BSNL): now also C30.1
- net at U2.21 (OUTNL): now also U2.23 (OUTPL), C30.2, C31.1, L2.1
- net at U2.24 (BSPL): now also C31.2
- net at U2.26 (BSNR): now also C29.2
- net at U2.27 (OUTNR): now also U2.29 (OUTPR), C28.1, C29.1, L1.1
- net at U2.30 (BSPR): now also C28.2
- net at U2.4 (RINP): now also C24.1
- net at U2.5 (RINN): now also C23.1
- net at U2.6 (PLIMIT): now also U2.7 (GVDD), C22.1, R12.1
- net at U2.8 (GAIN/SLV): now also R11.1, R12.2
- net at R40.1: now also C67.1, U12.6 (VCC)
- net at R49.1: now also U26.7 (OUTR)
- net SS 0: now reaches J1.1 (Pin_1)
- net SS 0: now also U3.1 (CS0/PS0)
- net SS 9: now reaches J1.10 (Pin_10)
- net SS 9: now also U3.15 (CS9/GPO1)
- net SS 10: now reaches J1.11 (Pin_11)
- net SS 10: now also U3.14 (CS10/GPO2)
- net SS 11: now reaches J1.12 (Pin_12)
- net SS 11: now also U3.13 (CS11/GPO3)
- net SS 12: now reaches J1.13 (Pin_13)
- net SS 12: now also U3.12 (CS12/GPO4)
- net SS 1: now reaches J1.2 (Pin_2)
- net SS 1: now also U3.2 (CS1/PS1)
- net SS 2: now reaches J1.3 (Pin_3)
- net SS 2: now also U3.3 (CS2/GUARD)
- net SS 3: now reaches J1.4 (Pin_4)
- net SS 3: now also U3.4 (CS3)
- net SS 4: now reaches J1.5 (Pin_5)
- net SS 4: now also U3.20 (CS4)
- net SS 5: now reaches J1.6 (Pin_6)
- net SS 5: now also U3.19 (CS5)
- net SS 6: now reaches J1.7 (Pin_7)
- net SS 6: now also U3.18 (CS6)
- net SS 7: now reaches J1.8 (Pin_8)
- net SS 7: now also U3.17 (CS7)
- net SS 8: now reaches J1.9 (Pin_9)
- net SS 8: now also U3.16 (CS8/GPO0)
- net at USB2.4 (CC1): now also C138.1, U32.C1 (CC1); no longer R1.1
- net IOFF 14: now reaches U3.10 (CS14/GPO6)
- net IOFF 14: now also J2.2 (Pin_2)
- net IOFF 13: now reaches U3.11 (CS13/GPO5)
- net IOFF 13: now also J2.1 (Pin_1)
- net SS SDA: now reaches U3.21 (I2CSDA)
- net SS SCL: now reaches U3.22 (I2CSCL)
- net SS XRES GPIO: now reaches U3.24 (~{XRES})
- net at U3.5 (CMOD): now also C97.1
- net at U3.6 (VCC): now also C96.1
- net IOFF 15: now reaches U3.9 (CS15/SH/~{HI})
- net IOFF 15: now also J2.3 (Pin_3)
- net I2C_SCL: no longer names the net of R31.1
- net I2C_SCL: now also C56.2, R32.2, U35.5 (FB)
- new net: R80.1, U21.16 (RIN-)
- new net: R79.2, R81.2, U21.17 (RIN+)
- new net: R76.2, R77.2, U21.4 (LIN+)
- new net: R78.1, U21.5 (LIN-)
- new net: U31.19 (LODRV), U34.4 (G)
- new net: C143.2, L12.1, U31.20 (PH), U33.1 (S), U33.2 (S), U33.3 (S), U34.5 (D), U34.6 (D), U34.7 (D), U34.8 (D), U34.9 (D)
- new net: C123.1, R20.1
- new net: C140.1, U31.10 (VREF), U31.4 (CE)
- new net: R66.1, R86.1, U31.11 (ISET1)
- new net: C154.1, R97.2, R98.1, U31.12 (VFB)
- new net: C155.2, C156.1, L12.2, R96.1, U31.14 (SRP)
- new net: R69.1, R87.1, U31.15 (ISET2)
- new net: R74.1, R88.1, U31.16 (ACSET)
- new net: C149.1, D28.1 (A), U31.18 (REGN)
- new net: C145.1, C146.2, Q2.1 (S), Q2.2 (S), Q2.3 (S), R93.1, U31.2 (ACP)
- new net: U31.21 (HIDRV), U33.4 (G)
- new net: C143.1, D28.3 (K), U31.22 (BTST)
- new net: R94.1, U31.23 (~{BATDRV})
- new net: C151.1, R91.2, U31.24 (VCC)
- new net: R89.2, U31.3 (~{ACDRV})
- new net: D29.1 (K), U31.5 (STAT1)
- new net: C157.1, R102.2, U31.6 (TS)
- new net: C141.1, U31.7 (TTC)
- new net: D31.1 (K), U31.8 (~{PG})
- new net: D30.1 (K), U31.9 (STAT2)
- new net: C186.2, C187.1, U16.26 (LDOO)
- new net: R60.1, R61.1, U19.6 (IN1+)
- new net: R47.1, U16.6 (OUTL)
- new net: C68.2, U12.7 (BOOT)
- new net: C75.1, C77.2, R51.2
- new net: R64.1, R67.2, U28.3 (IN2-)
- new net: R72.1, R75.2, U29.3 (IN2-)
- new net: C167.1, L14.1, U14.8 (SW)
- new net: C76.2, R50.2, U24.4 (IN2+)
- new net: C73.2, R28.1, U24.6 (IN1+)
- new net: D30.2 (A), R100.1
- new net: C69.2, R41.1, R42.2, U12.5 (FB)
- new net: C55.2, U35.7 (BOOT)
- new net: C180.1, L6.1, U15.2 (SW)
- new net: C180.2, U15.6 (BOOT)
- new net: R62.2, R63.1, U19.7 (IN1-)
- new net: C72.2, R27.1, R28.2
- new net: C84.2, C90.1, U26.26 (LDOO)
- new net: C110.1, L3.1, U30.29 (OUTPR)
- new net: R23.1, U30.16 (SYNC)
- new net: C131.2, R26.1
- new net: C122.2, R19.2
- new net: C74.2, C76.1, R29.2
- new net: R102.1, R103.1, R104.2, R105.1
- new net: R70.2, R71.1, U22.3 (IN2-)
- new net: R68.1, U22.4 (IN2+)
- new net: U22.7 (IN1-), U22.8 (OUT1)
- new net: C112.1, L10.1, U30.23 (OUTPL)
- new net: C112.2, U30.24 (BSPL)
- new net: R44.1, R45.2, U15.4 (FB)
- new net: C129.2, R24.2
- new net: C191.1, U16.2 (CAPP)
- new net: C191.2, U16.4 (CAPM)
- new net: R5.1, R59.2, U19.3 (IN2-)
- new net: C142.1, Q1.1 (S), Q1.2 (S), Q1.3 (S), Q2.5 (D), R90.1, R91.1
- new net: C142.2, Q1.4 (G), Q2.4 (G), R89.1, R90.2
- new net: C88.1, U26.10 (VCOM/DEMP)
- new net: R46.1, U16.7 (OUTR)
- new net: C78.2, C79.2, R52.1, R53.1, R53.2, U25.4 (IN2+)
- new net: D31.2 (A), R101.1
- new net: R4.1, U4.7 (OUTR)
- new net: R16.1, R9.2, U30.8 (GAIN/SLV)
- new net: C107.1, U30.10 (LINP)
- new net: C124.1, U30.11 (LINN)
- new net: C113.1, U30.20 (BSNL)
- new net: C113.2, L11.1, U30.21 (OUTNL)
- new net: C111.2, U30.26 (BSNR)
- new net: C111.1, L7.1, U30.27 (OUTNR)
- new net: C110.2, U30.30 (BSPR)
- new net: C105.1, U30.4 (RINP)
- new net: C106.1, U30.5 (RINN)
- new net: C50.1, R9.1, U30.6 (PLIMIT), U30.7 (GVDD)
- new net: R73.1, U29.4 (IN2+)
- new net: C192.1, U16.10 (VCOM/DEMP)
- new net: C188.2, U16.5 (VNEG)
- new net: C36.2, R14.2
- new net: U20.2 (OUT2), U20.3 (IN2-)
- new net: D29.2 (A), R99.1
- new net: C10.2, C16.1, U4.26 (LDOO)
- new net: C166.1, R37.1, U14.6 (VCC)
- new net: C85.2, U26.5 (VNEG)
- new net: C130.1, R25.1
- new net: C158.1, L13.1, U13.8 (SW)
- new net: C2.1, U4.2 (CAPP)
- new net: C2.2, U4.4 (CAPM)
- new net: U18.2 (OUT2), U18.3 (IN2-)
- new net: R6.1, U19.4 (IN2+)
- new net: R65.1, U28.4 (IN2+)
- new net: C37.1, R15.1
- new net: R52.2, U25.7 (IN1-), U25.8 (OUT1)
- new net: R3.1, U4.6 (OUTL)
- new net: C14.1, U4.10 (VCOM/DEMP)
- new net: C11.2, U4.5 (VNEG)
- new net: C168.2, R38.1, R39.2, U14.5 (FB)
- new net: C75.2, R30.2, U25.6 (IN1+)
- new net: C144.1, R92.1
- new net: C148.1, Q3.4 (G), R94.2, R95.2
- new net: C167.2, U14.7 (BOOT)
- new net: C81.1, U26.2 (CAPP)
- new net: C81.2, U26.4 (CAPM)
- new net: C158.2, U13.7 (BOOT)
- new net: R43.1, R44.2
- new net +3.3VA: C12.1, C13.1, C17.1, C189.1, C190.1, C193.1, C194.1, C3.1, C82.1, C86.1, C87.1, C91.1, U16.1 (CPVDD), U16.25 (XSMT), U16.8 (AVDD), U26.1 (CPVDD), U26.25 (XSMT), U26.8 (AVDD), U4.1 (CPVDD), U4.25 (XSMT), U4.8 (AVDD)
- new net -12V: C133.2, C136.2, C178.2, C179.2, C181.2, C182.2, C183.2, C19.2, C4.2, C41.2, C46.2, C48.2, C51.2, C53.2, C6.2, C8.2, R45.1, U1.5 (VCC-), U15.1 (GND), U18.5 (VCC-), U19.5 (VCC-), U20.5 (VCC-), U21.1 (LVCC-), U21.20 (RVCC-), U22.5 (VCC-), U24.5 (VCC-), U25.5 (VCC-), U28.5 (VCC-), U29.5 (VCC-)
- new net ADR1 HEADPHONE: U4.24 (ADR1/MISO/FMT)
- new net ADR1 SPEAKER: U16.24 (ADR1/MISO/FMT)
- new net ADR1 STEREO OUT: U26.24 (ADR1/MISO/FMT)
- new net ADR2 HEADPHONE: U4.16 (ADR2/GPIO2/DOUT)
- new net ADR2 SPEAKER: U16.16 (ADR2/GPIO2/DOUT)
- new net ADR2 STEREO OUT: U26.16 (ADR2/GPIO2/DOUT)
- new net BCK HEADPHONE: U4.21 (BCK)
- new net BCK SPEAKER: U16.21 (BCK)
- new net BCK STEREO OUT: U26.21 (BCK)
- new net DIN HEADPHONE: U4.22 (DIN)
- new net DIN SPEAKER: U16.22 (DIN)
- new net DIN STEREO OUT: U26.22 (DIN)
- new net GPIO3 HEADPHONE: U4.15 (GPIO3/AGNS)
- new net GPIO3 SPEAKER: U16.15 (GPIO3/AGNS)
- new net GPIO3 STEREO OUT: U26.15 (GPIO3/AGNS)
- new net GPIO4 HEADPHONE: U4.14 (GPIO4/MAST)
- new net GPIO4 SPEAKER: U16.14 (GPIO4/MAST)
- new net GPIO4 STEREO OUT: U26.14 (GPIO4/MAST)
- new net GPIO5 HEADPHONE: U4.13 (GPIO5/ATT0)
- new net GPIO5 SPEAKER: U16.13 (GPIO5/ATT0)
- new net GPIO5 STEREO OUT: U26.13 (GPIO5/ATT0)
- new net GPIO6 HEADPHONE: U4.19 (GPIO6/FLT)
- new net GPIO6 SPEAKER: U16.19 (GPIO6/FLT)
- new net GPIO6 STEREO OUT: U26.19 (GPIO6/FLT)
- new net HEADPHONE AMP L: AUDIO1.2, U21.2 (LOUT)
- new net HEADPHONE AMP R: AUDIO1.3, U21.19 (ROUT)
- new net HEADPHONE BUFF L N: R67.1, R78.2, U28.2 (OUT2)
- new net HEADPHONE BUFF L P: R64.2, R76.1, U28.7 (IN1-), U28.8 (OUT1)
- new net HEADPHONE BUFF R N: R75.1, R80.2, U29.2 (OUT2)
- new net HEADPHONE BUFF R P: R72.2, R79.1, U29.7 (IN1-), U29.8 (OUT1)
- new net HEADPHONE DAC L: C18.1, R3.2, U28.6 (IN1+)
- new net HEADPHONE DAC R: C80.1, R4.2, U29.6 (IN1+)
- new net HEADPHONE GPIO L: AUDIO1.6, R84.1
- new net HEADPHONE GPIO R: AUDIO1.7, R85.1
- new net INT_N USB: R58.2, U32.B2 (INT_N)
- new net LRCK HEADPHONE: U4.23 (LRCK)
- new net LRCK SPEAKER: U16.23 (LRCK)
- new net LRCK STEREO OUT: U26.23 (LRCK)
- new net MONO BUFF: R7.2, R8.1, U18.7 (IN1-), U18.8 (OUT1), U23.9 (NC1)
- new net MUTE TWEET/WOOF: R18.1, U30.12 (MUTE)
- new net SCK HEADPHONE: U4.20 (SCK)
- new net SCK SPEAKER: U16.20 (SCK)
- new net SCK STEREO OUT: U26.20 (SCK)
- new net SCL HEADPHONE: U4.12 (SCL/MC/ATT1)
- new net SCL SPEAKER: U16.12 (SCL/MC/ATT1)
- new net SCL STEREO OUT: U26.12 (SCL/MC/ATT1)
- new net SCL USB: R2.1, U32.B3 (SCL)
- new net SDA HEADPHONE: U4.11 (SDA/MOSI/ATT2)
- new net SDA SPEAKER: U16.11 (SDA/MOSI/ATT2)
- new net SDA STEREO OUT: U26.11 (SDA/MOSI/ATT2)
- new net SDA USB: R1.2, U32.C3 (SDA)
- new net SPEAKER DAC L: C196.1, R21.1, R47.2
- new net SPEAKER DAC R: C195.1, R22.2, R46.2
- new net SPEAKER SUM BUFF: C74.1, C77.1, R21.2, R22.1, R27.2, U20.7 (IN1-), U20.8 (OUT1)
- new net STEREO BUFF L: U1.7 (IN1-), U1.8 (OUT1), U23.2 (NO1)
- new net STEREO DAC L: R7.1, U1.6 (IN1+)
- new net STEREO DAC R: R8.2, U1.4 (IN2+)
- new net STEREO OUT DAC L: C92.1, R48.2
- new net STEREO OUT DAC R: C93.1, R49.2
- new net SUB AMP N: C32.1, C35.1, L2.2, R15.2
- new net SUB AMP P: C33.2, C34.2, L1.2, R14.1
- new net SUB SUM BUFF: C24.2, R5.2, U24.7 (IN1-), U24.8 (OUT1)
- new net SUB SUM BUFF N: C23.2, R59.1, U19.2 (OUT2)
- new net TWEET AMP N: C119.1, C121.1, L7.2, R20.2
- new net TWEET AMP P: C118.2, C120.2, L3.2, R19.1
- new net TWEET SUM BUFF: C105.2, R63.2, U24.2 (OUT2), U24.3 (IN2-)
- new net TWEET SUM BUFF N: C106.2, R62.1, U19.8 (OUT1)
- new net WOOF AMP N: C126.1, C128.1, L11.2, R25.2
- new net WOOF AMP P: C125.2, C127.2, L10.2, R24.1
- new net WOOF SUM BUFF: C107.2, R71.2, U25.2 (OUT2), U25.3 (IN2-)
- new net WOOF SUM BUFF N: C124.2, R70.1, U22.2 (OUT2)
- new net /SD TWEET/WOOF: R17.2, U30.2 (SDZ), U30.3 (FAULTZ)
- no-connect marks 3 -> 27
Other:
- note added: "Connect int a gpio exti"
- note removed: "Audio Amplifiers"
- note removed: "DAC"
- note removed: "If using thermistor, remove R43"
- note removed: "Touch Pad"
- note removed: "Usb Power outlet / Coding"
- moved on the sheet: C1, CN1, CN2, CN3, Card1, D1, D10, D11, D12, D13, D14, D15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

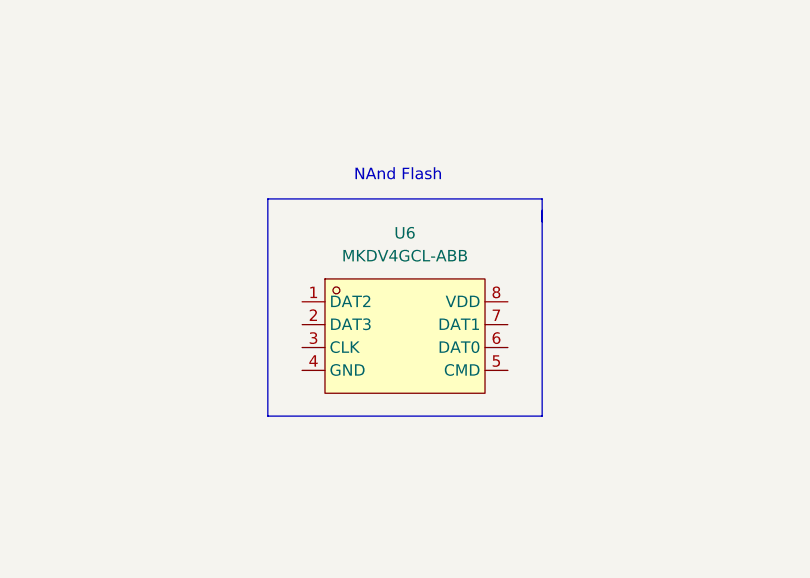
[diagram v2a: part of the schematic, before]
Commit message: g
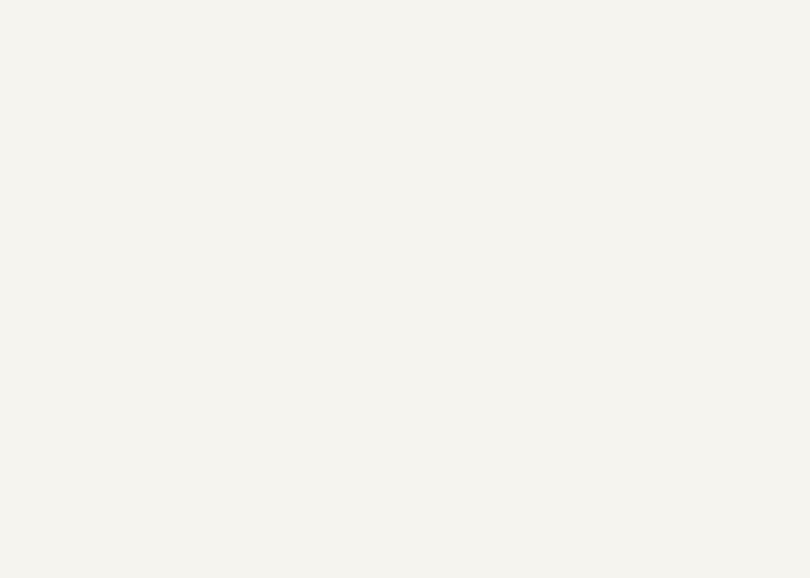
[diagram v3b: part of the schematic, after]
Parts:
- removed U6: MKDV4GCL-ABB, lcsc:LGA-8_L6.0-W8.0-P1.27-TL, symbol lcsc:MKDV4GCL-ABB
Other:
- note removed: "NAnd Flash"
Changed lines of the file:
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@@
 		)
 	)
-	(text "NAnd Flash"
-		(exclude_from_sim no)
-		(at 1071.118 378.46 0)
-		(effects
-			(font
-				(size 1.27 1.27)
-			)
-		)
-	)
 	(text "Function Knob"
 		(exclude_from_sim no)
@@
 		)
 	)
-	(polyline
-		(pts
-			(xy 1056.64 405.13) (xy 1056.64 381)
-		)
-		(stroke
-			(width 0)
-			(type default)
-		)
-	)
 	(wire
 		(pts
@@
 		)
 	)
-	(polyline
-		(pts
-			(xy 1056.64 381) (xy 1087.12 381)
-		)
-		(stroke
-			(width 0)
-			(type default)
-		)
-	)
 	(wire
 		(pts
@@
 		)
 	)
-	(polyline
-		(pts
-			(xy 1087.12 382.27) (xy 1087.12 405.13)
-		)
-		(stroke
-			(width 0)
-			(type default)
-		)
-	)
 	(wire
 		(pts
@@
 		)
 	)
-	(polyline
-		(pts
-			(xy 1087.12 381) (xy 1087.12 383.54)
-		)
-		(stroke
-			(width 0)
-			(type default)
-		)
-	)
 	(wire
 		(pts
@@
 		)
 	)
-	(polyline
-		(pts
-			(xy 1087.12 405.13) (xy 1056.64 405.13)
-		)
-		(stroke
-			(width 0)
-			(type default)
-		)
-	)
 	(wire
 		(pts
@@
 					(unit 1)
 				)
-			)
-		)
-	)
-	(symbol
-		(lib_id "lcsc:MKDV4GCL-ABB")
-		(at 1071.88 396.24 0)
-		(unit 1)
-		(exclude_from_sim no)
-		(in_bom yes)
-		(on_board yes)
-		(dnp no)
-		(fields_autoplaced yes)
-		(property "Reference" "U6"
-			(at 1071.88 384.81 0)
-			(effects
-				(font
-					(size 1.27 1.27)
-				)
-			)
-		)
-		(property "Value" "MKDV4GCL-ABB"
-			(at 1071.88 387.35 0)
-			(effects
-				(font
-					(size 1.27 1.27)
-				)
-			)
-		)
-		(property "Footprint" "lcsc:LGA-8_L6.0-W8.0-P1.27-TL"
-			(at 1071.88 407.67 0)
-			(effects
-				(font
-					(size 1.27 1.27)
-				)
-				(hide yes)
-			)
-		)
-		(property "Datasheet" ""
-			(at 1071.88 396.24 0)
-			(effects
-				(font
-					(size 1.27 1.27)
-				)
-				(hide yes)
-			)
-		)
-		(property "Description" ""
-			(at 1071.88 396.24 0)
-			(effects
-				(font
-					(size 1.27 1.27)
-				)
-				(hide yes)
-			)
-		)
-		(property "LCSC Part" "C7500178"
-			(at 1071.88 410.21 0)
-			(effects
-				(font
-					(size 1.27 1.27)
-				)
-				(hide yes)
-			)
-		)
-		(pin "1"
-		)
-		(pin "6"
-		)
-		(pin "5"
-		)
-		(pin "3"
-		)
-		(pin "8"
-		)
-		(pin "4"
-		)
-		(pin "7"
-		)
-		(pin "2"
-		)
-		(instances
-			(project ""
-				(path "/0dd47ee7-841f-4fd7-9fd1-ca99fc50fdde"
-					(reference "U6")
-					(unit 1)
-				)
